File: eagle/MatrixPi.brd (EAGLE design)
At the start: 85 x 56 mm, 17 parts, among them U2 28-SOIC

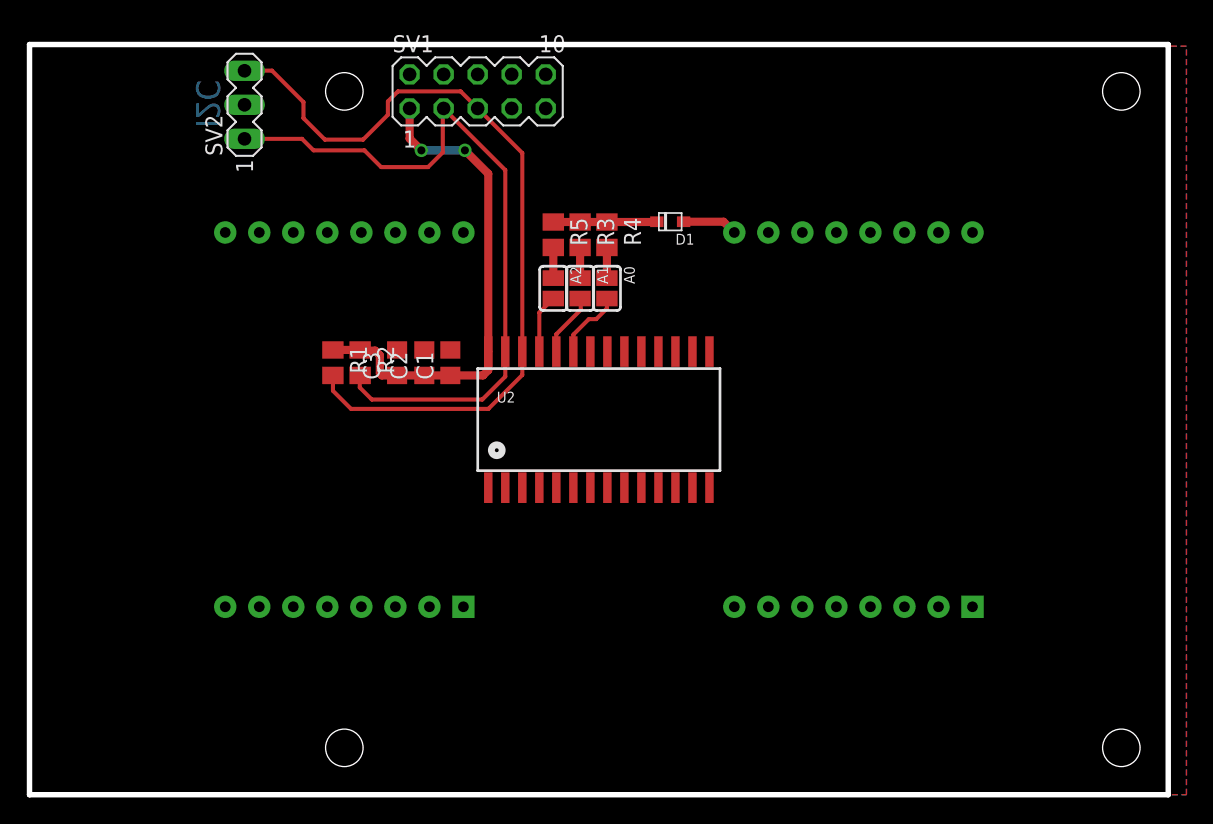
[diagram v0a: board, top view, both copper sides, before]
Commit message: Board revisions
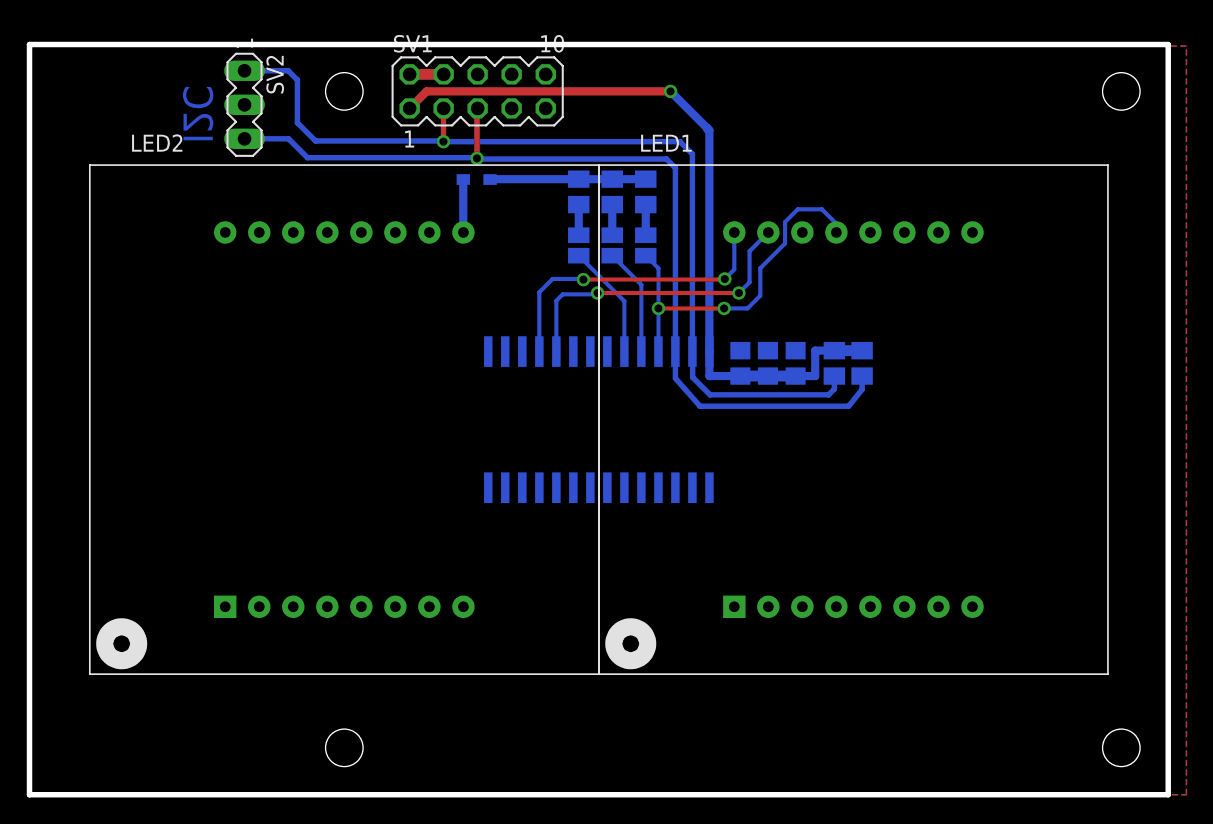
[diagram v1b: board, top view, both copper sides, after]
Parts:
- moved R1 39.5 mm to (62.1, 32.2), flipped to the bottom
- moved R2 35.4 mm to (60.1, 32.2), flipped to the bottom
- moved C3 29.8 mm to (57.2, 32.2), flipped to the bottom
- moved C2 25.7 mm to (55.1, 32.2), flipped to the bottom
- moved C1 21.7 mm to (53.1, 32.2), flipped to the bottom
- moved D1 14.8 mm to (33.4, 45.9), flipped to the bottom
- moved A2 7.61 mm to (46.0, 41.0), flipped to the bottom
- moved R5 7.61 mm to (46.0, 45.0), flipped to the bottom
- moved A1 4.00 mm to (43.5, 41.0), flipped to the bottom
- moved R3 4.00 mm to (43.5, 45.0), flipped to the bottom
- moved A0 3.83 mm to (41.0, 41.0), flipped to the bottom
- moved R4 3.83 mm to (41.0, 45.0), flipped to the bottom
- flipped LED1 to the top
- flipped LED2 to the top
- turned SV2 to 270 degrees
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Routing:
- net N$23: track 0.00 -> 23.7 mm, vias 0 -> 2
- net A2: track 4.39 -> 27.1 mm, vias 0 -> 2
- net N$22: track 0.00 -> 22.5 mm, vias 0 -> 2
- net VDD: track 37.2 -> 55.8 mm, vias 2 -> 1
- net SDA: track 54.2 -> 69.3 mm, vias 0 -> 1
- net SCL: track 61.0 -> 69.0 mm, vias 0 -> 1
- net N$16: track 7.74 -> 11.7 mm
- net A1: track 4.73 -> 8.06 mm
- net A0: track 5.32 -> 8.57 mm
- net +5V: track 0.00 -> 2.54 mm
